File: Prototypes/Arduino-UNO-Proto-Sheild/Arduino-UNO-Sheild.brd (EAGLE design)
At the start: 160 x 100 mm, 1 part, among them J1 ARDUINO_R3_SHIELD

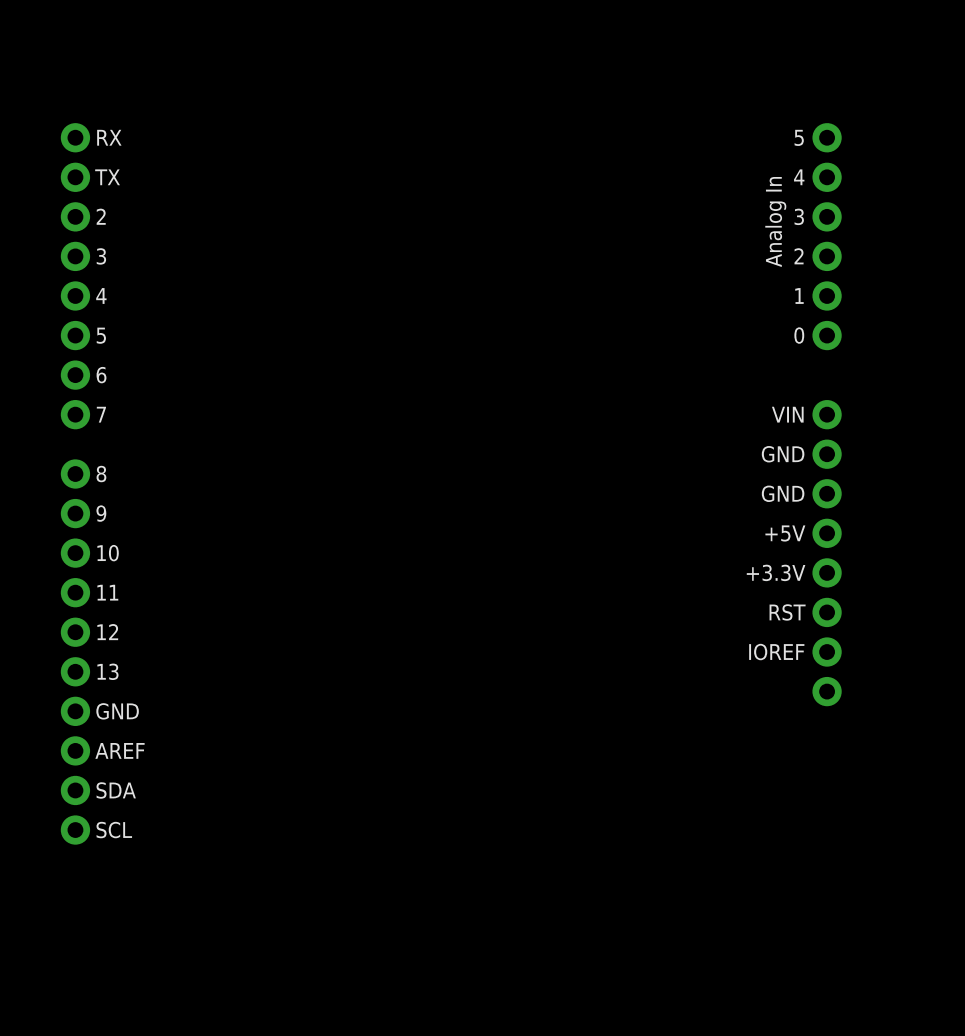
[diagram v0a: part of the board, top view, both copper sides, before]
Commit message: Fixes
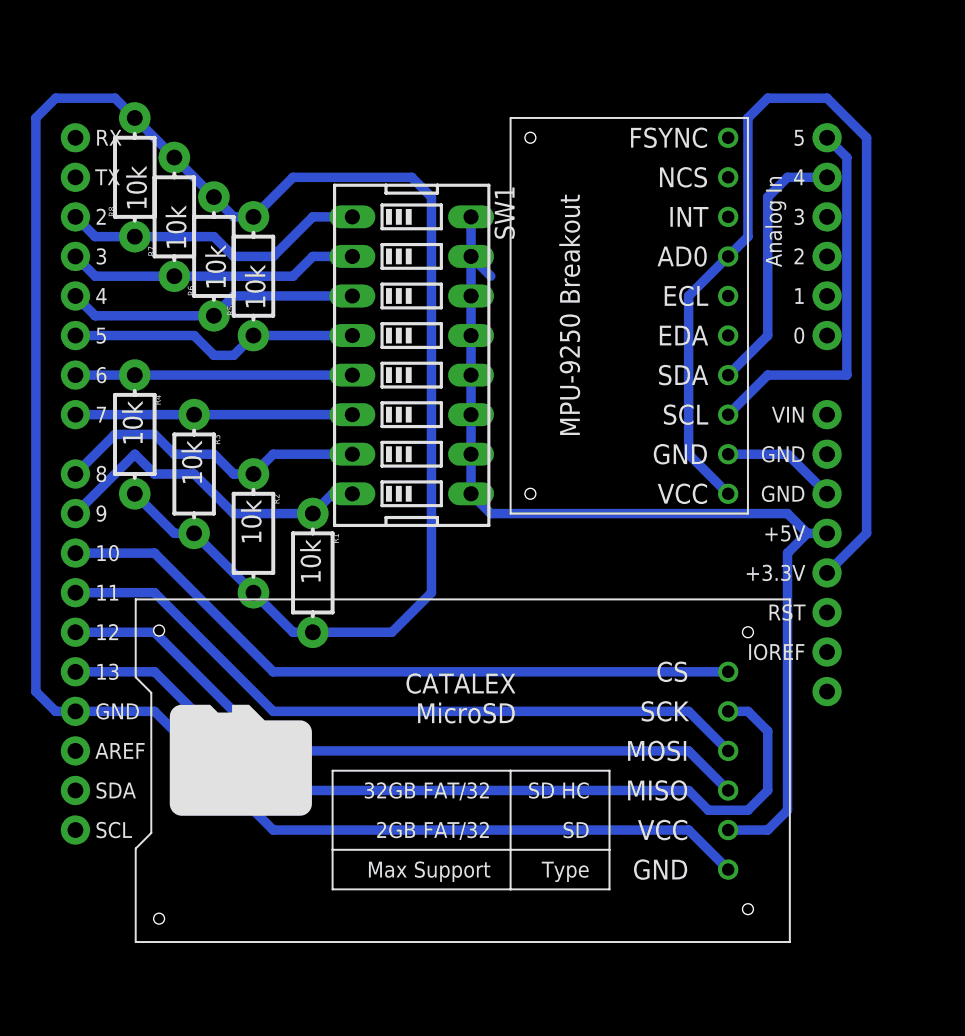
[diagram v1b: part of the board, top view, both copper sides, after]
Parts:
- added R1, R2, R3, R4, R5, R6, R7, R8: 10k, SparkFun-Passives:AXIAL-0.3-KIT
- added SW1: (no value), SparkFun-Electromechanical:DIPSWITCH-08
- added U$1: CATALEX-MICROSD-BREAKOUT, Modules:CATALEX-MICROSD-BREAKOUT
- added U$2: MPU-9250-BREAKOUT, Modules:MPU-9250-BREAKOUT
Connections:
- new net N$1: J1.A4, U$2.SDA
- new net N$10: J1.D9, R1.P$1, SW1.8
- new net N$11: J1.D8, R2.P$1, SW1.7
- new net N$12: J1.D7, R3.P$1, SW1.6
- new net N$13: J1.D6, R4.P$1, SW1.5
- new net N$14: J1.D5, R5.P$1, SW1.4
- new net N$15: J1.D4, R6.P$1, SW1.3
- new net N$16: J1.D3, R7.P$1, SW1.2
- new net N$17: J1.D2, R8.P$1, SW1.1
- new net N$18: J1.5V, SW1.10, SW1.11, SW1.12, SW1.13, SW1.14, SW1.15, SW1.16, SW1.9, U$1.VCC
- new net N$2: J1.A5, U$2.SCL
- new net N$20: J1.GND@2, R1.P$2, R2.P$2, R3.P$2, R4.P$2, R5.P$2, R6.P$2, R7.P$2, R8.P$2, U$1.GND
- new net N$3: J1.3.3V, U$2.AD0, U$2.VCC
- new net N$4: J1.GND@0, U$2.GND
- new net N$6: J1.D10, U$1.CS
- new net N$7: J1.D13, U$1.SCK
- new net N$8: J1.D11, U$1.MOSI
- new net N$9: J1.D12, U$1.MISO
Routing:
- net N$20: track 0.00 -> 165.9 mm
- net N$18: track 0.00 -> 66.1 mm
- net N$3: track 0.00 -> 65.0 mm
- net N$7: track 0.00 -> 55.5 mm
- net N$9: track 0.00 -> 46.1 mm
- net N$8: track 0.00 -> 46.1 mm
- net N$6: track 0.00 -> 45.1 mm
- net N$2: track 0.00 -> 24.4 mm
- net N$10: track 0.00 -> 21.5 mm
- net N$11: track 0.00 -> 20.4 mm
- net N$17: track 0.00 -> 19.9 mm
- net N$16: track 0.00 -> 18.8 mm
- net N$15: track 0.00 -> 18.8 mm
- net N$14: track 0.00 -> 18.8 mm
- net N$13: track 0.00 -> 17.8 mm
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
